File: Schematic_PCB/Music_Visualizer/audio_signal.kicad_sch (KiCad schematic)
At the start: 16 parts, among them J1 NMJ4HCD2, J3 Screw_Terminal_01x02, J4 NMJ4HCD2, J5 Screw_Terminal_01x02, U2 LM324, U3 LM324

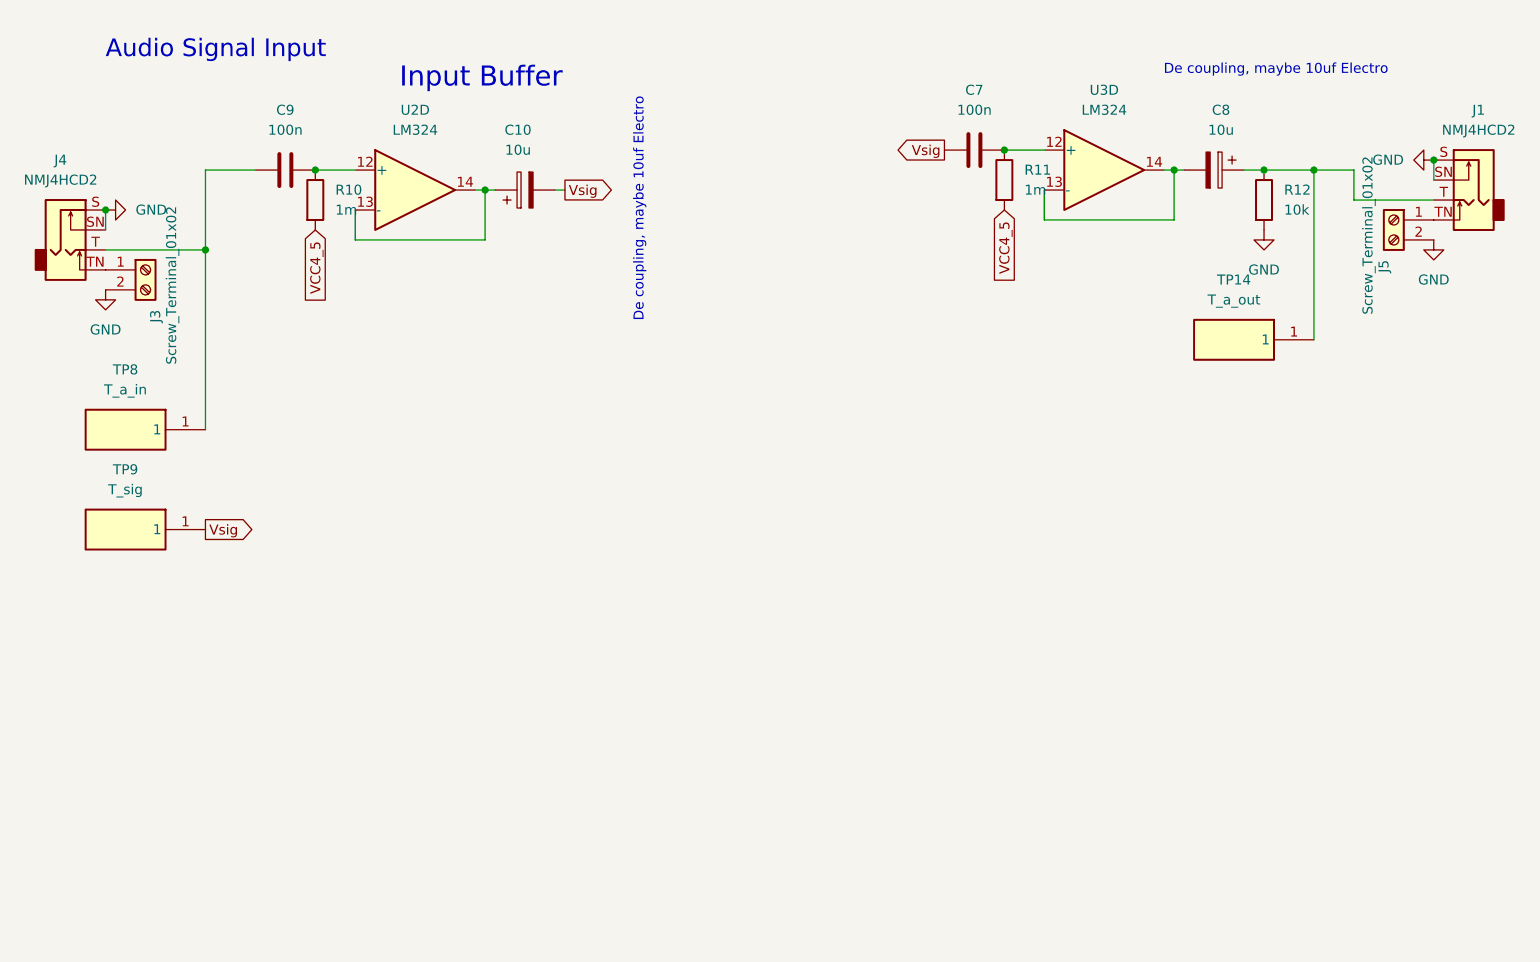
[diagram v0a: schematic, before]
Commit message: In-Out switch
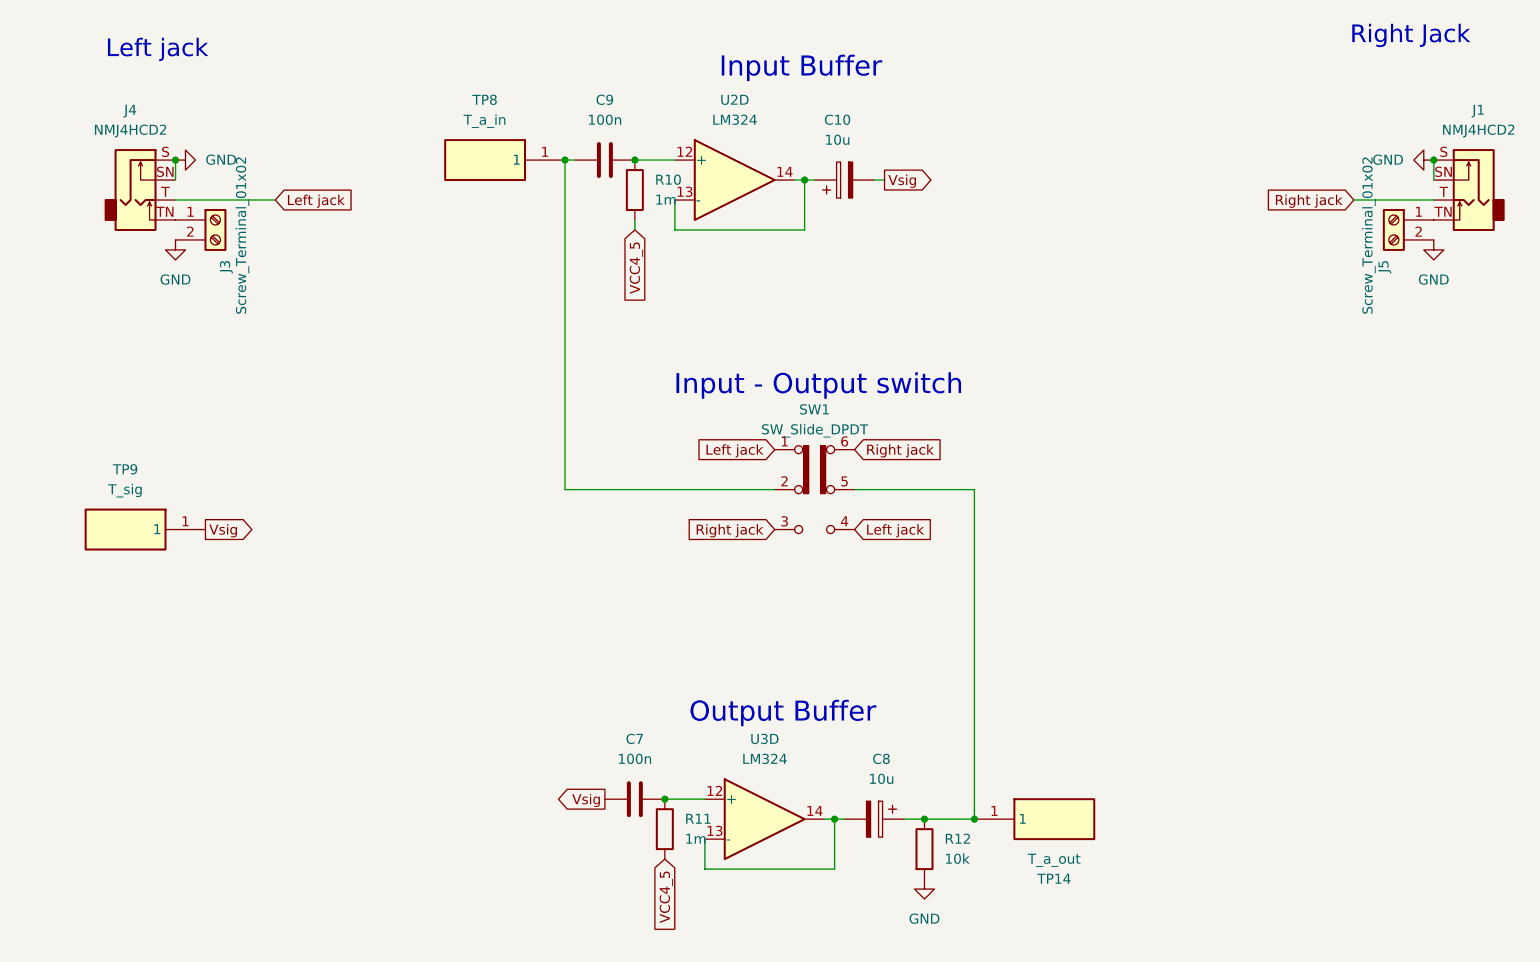
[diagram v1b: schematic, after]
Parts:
- added SW1: SW_Slide_DPDT, Button_Switch_THT:SW_CK_JS202011CQN_DPDT_Straight, symbol Switch:SW_Slide_DPDT
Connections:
- net at C8.1, R12.1, TP14.1: now also SW1.5 (B); no longer J1.T
- net at C9.1, TP8.1: now also SW1.2 (B); no longer J4.T
- new net Left jack: J4.T, SW1.1 (A), SW1.4 (A)
- new net Right jack: J1.T, SW1.3 (C), SW1.6 (C)
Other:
- note added: "Input - Output switch"
- note added: "Left jack"
- note added: "Output Buffer"
- note added: "Right Jack"
- note removed: "Audio Signal Input"
- note removed: "De coupling, maybe 10uf Electro"
- moved on the sheet: C10, C7, C8, C9, J3, J4, R10, R11, R12, TP14, TP8, U2D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
